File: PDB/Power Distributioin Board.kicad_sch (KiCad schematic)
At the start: 29 parts, among them J1 INPUT, J2 3.3v, J3 1.8v, J4 5v, U2 MAX16910, U3 MAX16910, U4 MAX16910

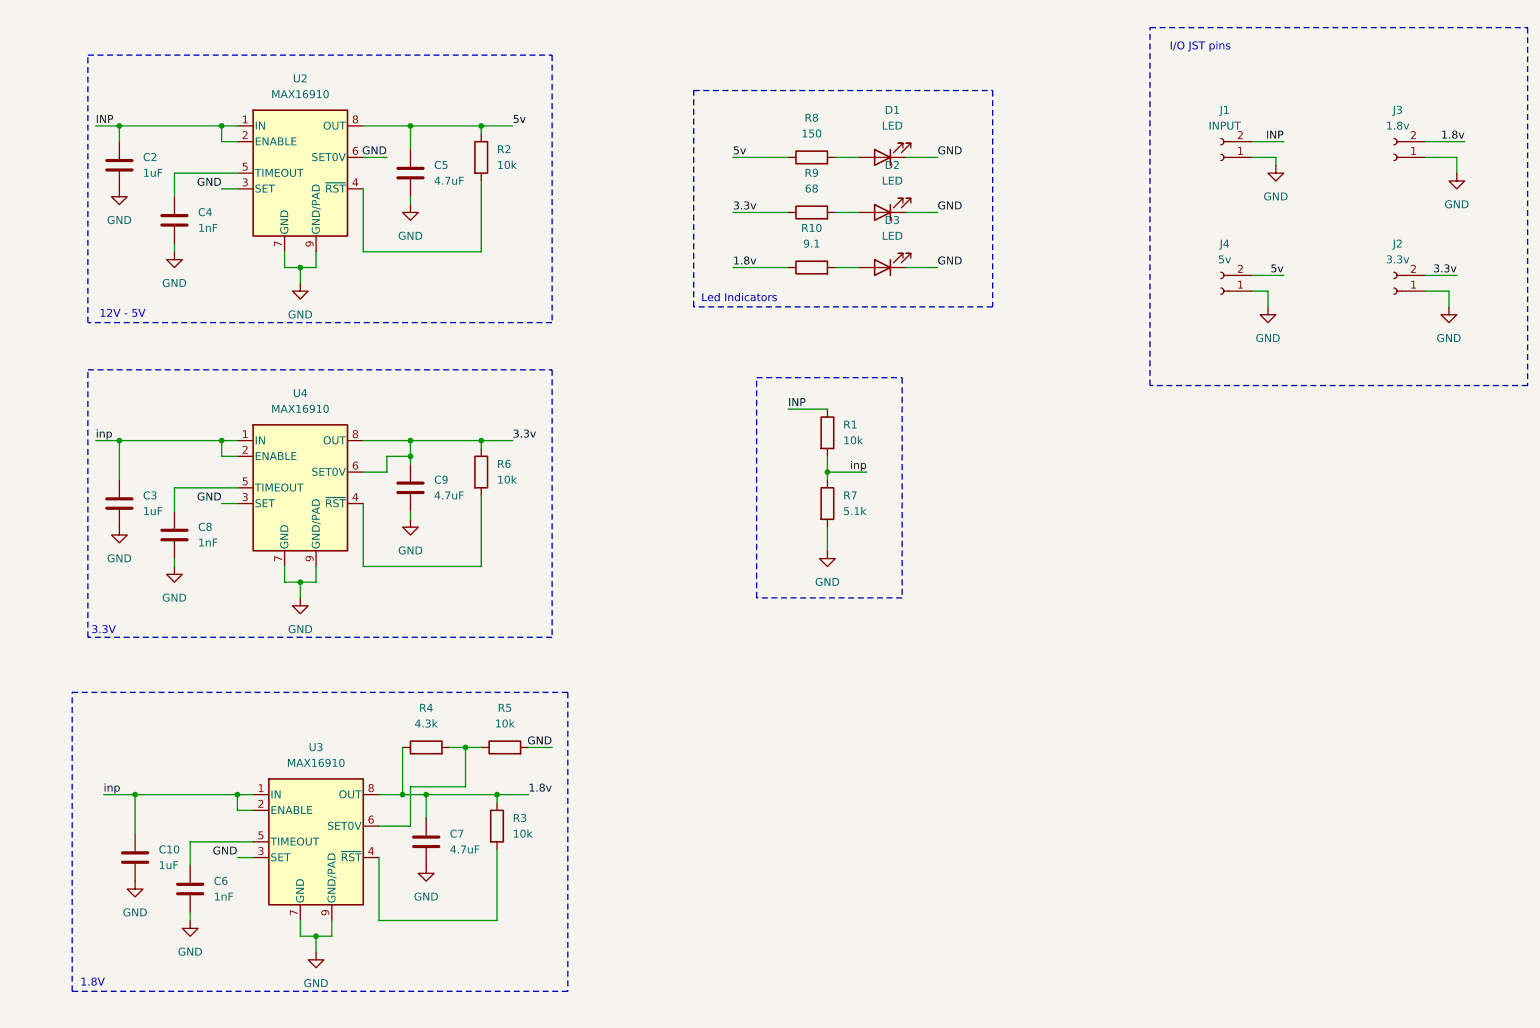
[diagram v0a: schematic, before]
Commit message: Pdb
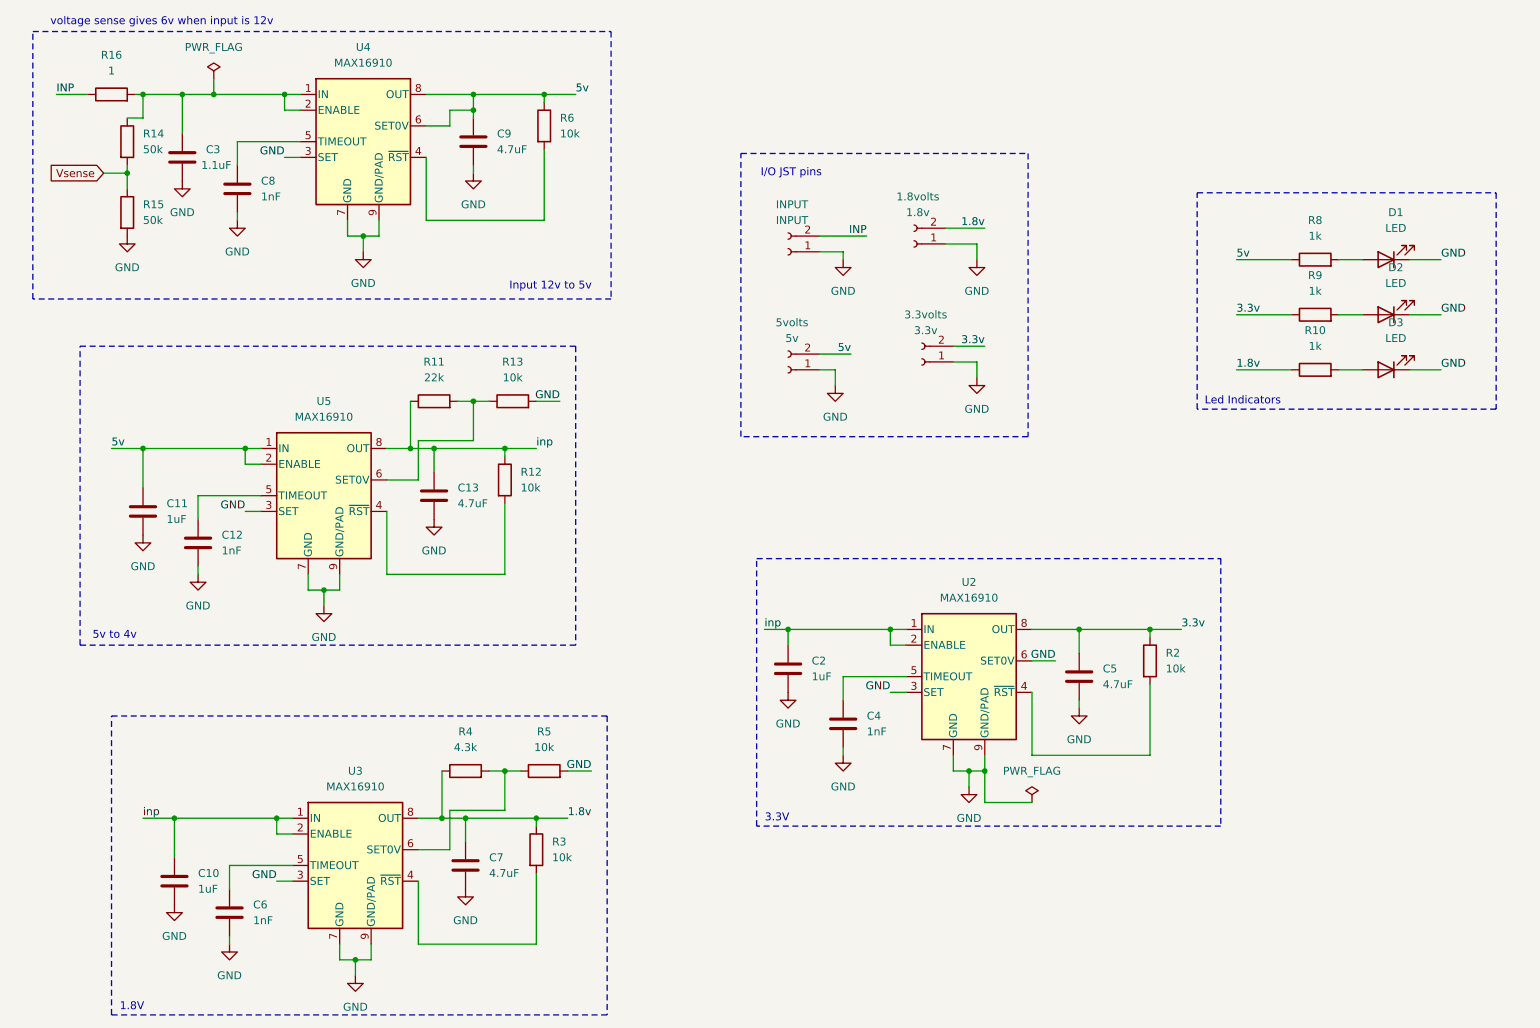
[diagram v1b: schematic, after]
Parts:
- removed R1: 10k, Resistor_SMD:R_0805_2012Metric, symbol Device:R
- removed R7: 5.1k, Resistor_SMD:R_0805_2012Metric, symbol Device:R
- added C11: 1uF, Capacitor_SMD:C_0805_2012Metric, symbol Device:C
- added C12: 1nF, Capacitor_SMD:C_0805_2012Metric, symbol Device:C
- added C13: 4.7uF, Capacitor_SMD:C_0805_2012Metric, symbol Device:C
- added R11: 22k, Resistor_SMD:R_0805_2012Metric, symbol Device:R
- added R12, R13: 10k, Resistor_SMD:R_0805_2012Metric, symbol Device:R
- added R14, R15: 50k, Resistor_SMD:R_0805_2012Metric, symbol Device:R
- added R16: 1, Resistor_SMD:R_0805_2012Metric, symbol Device:R
- added U5: MAX16910, maxy:SON65P300X300X80-9N, symbol Regulator_Linear:MAX16910
- C3: value 1uF -> 1.1uF
- R10: value 9.1 -> 1k
- R8: value 150 -> 1k
- R9: value 68 -> 1k
- renumbered J3 to 1.8volts, J2 to 3.3volts, J4 to 5volts, J1 to INPUT
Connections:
- net 3.3v: now also C5.1, R2.1, U2.8 (OUT); no longer C9.1, R6.1, U4.6 (SET0V), U4.8 (OUT)
- net 5v: now also C9.1, R6.1, U4.6 (SET0V), U4.8 (OUT), C11.1, U5.1 (IN), U5.2 (ENABLE); no longer C5.1, R2.1, U2.8 (OUT)
- net GND: now also C11.2, C12.2, C13.2, R13.2, R15.2, U5.3 (SET), U5.7 (GND), U5.9 (GND/PAD)
- net INP: now also R16.1; no longer C2.1, U2.1 (IN), U2.2 (ENABLE)
- net inp: now also C2.1, U2.1 (IN), U2.2 (ENABLE), C13.1, R11.1, R12.1, U5.8 (OUT); no longer C3.1, U4.1 (IN), U4.2 (ENABLE)
- new net: R11.2, R13.1, U5.6 (SET0V)
- new net: R12.2, U5.4 (~{RST})
- new net: C12.1, U5.5 (TIMEOUT)
- new net: C3.1, R14.1, R16.2, U4.1 (IN), U4.2 (ENABLE)
- new net Vsense: R14.2, R15.1
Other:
- note added: "5v to 4v"
- note added: "Input 12v to 5v"
- note added: "voltage sense gives 6v when input is 12v"
- note removed: "12V - 5V"
- moved on the sheet: 1.8volts, 3.3volts, 5volts, C10, C2, C3, C4, C5, C6, C7, C8, C9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
